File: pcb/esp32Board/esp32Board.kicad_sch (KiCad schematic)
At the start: 35 parts, among them J1 ESPProgJTAG_RX, J10 USB_C_Receptacle_USB2.0, J11 Conn_01x14_Female, J3 ESPProgUART_RX, J4 CAN, J5 UART2, J6 I2C, J7 InputOnly, J8 PWR, J9 GND, SW1 SW_Push, SW2 SW_Push_SPDT, SW3 SW_Push_SPDT, SW4 SW_Push_SPDT, U1 ESP32-WROOM-32D, U3 XC6209

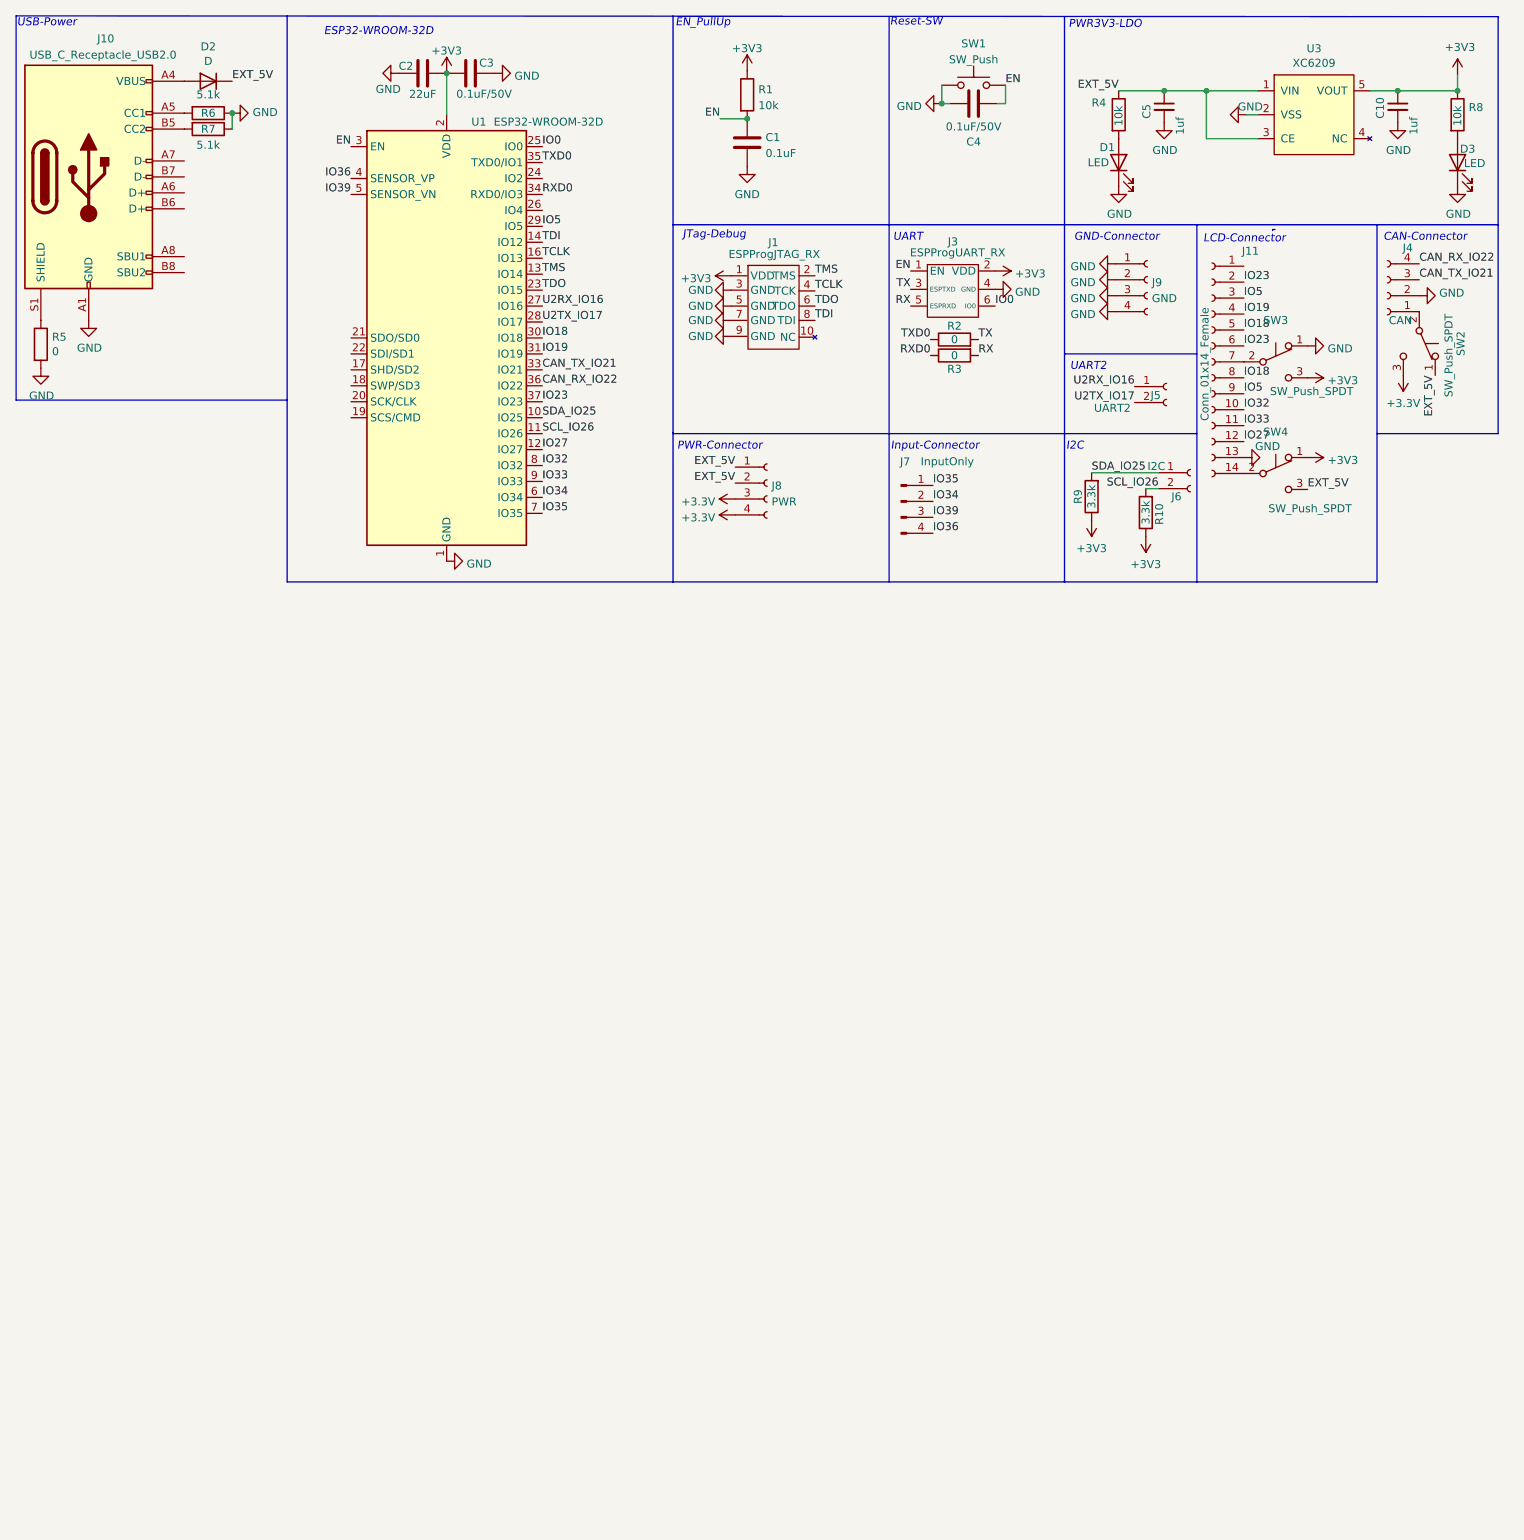
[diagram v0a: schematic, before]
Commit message: 改成竖的，论文好看
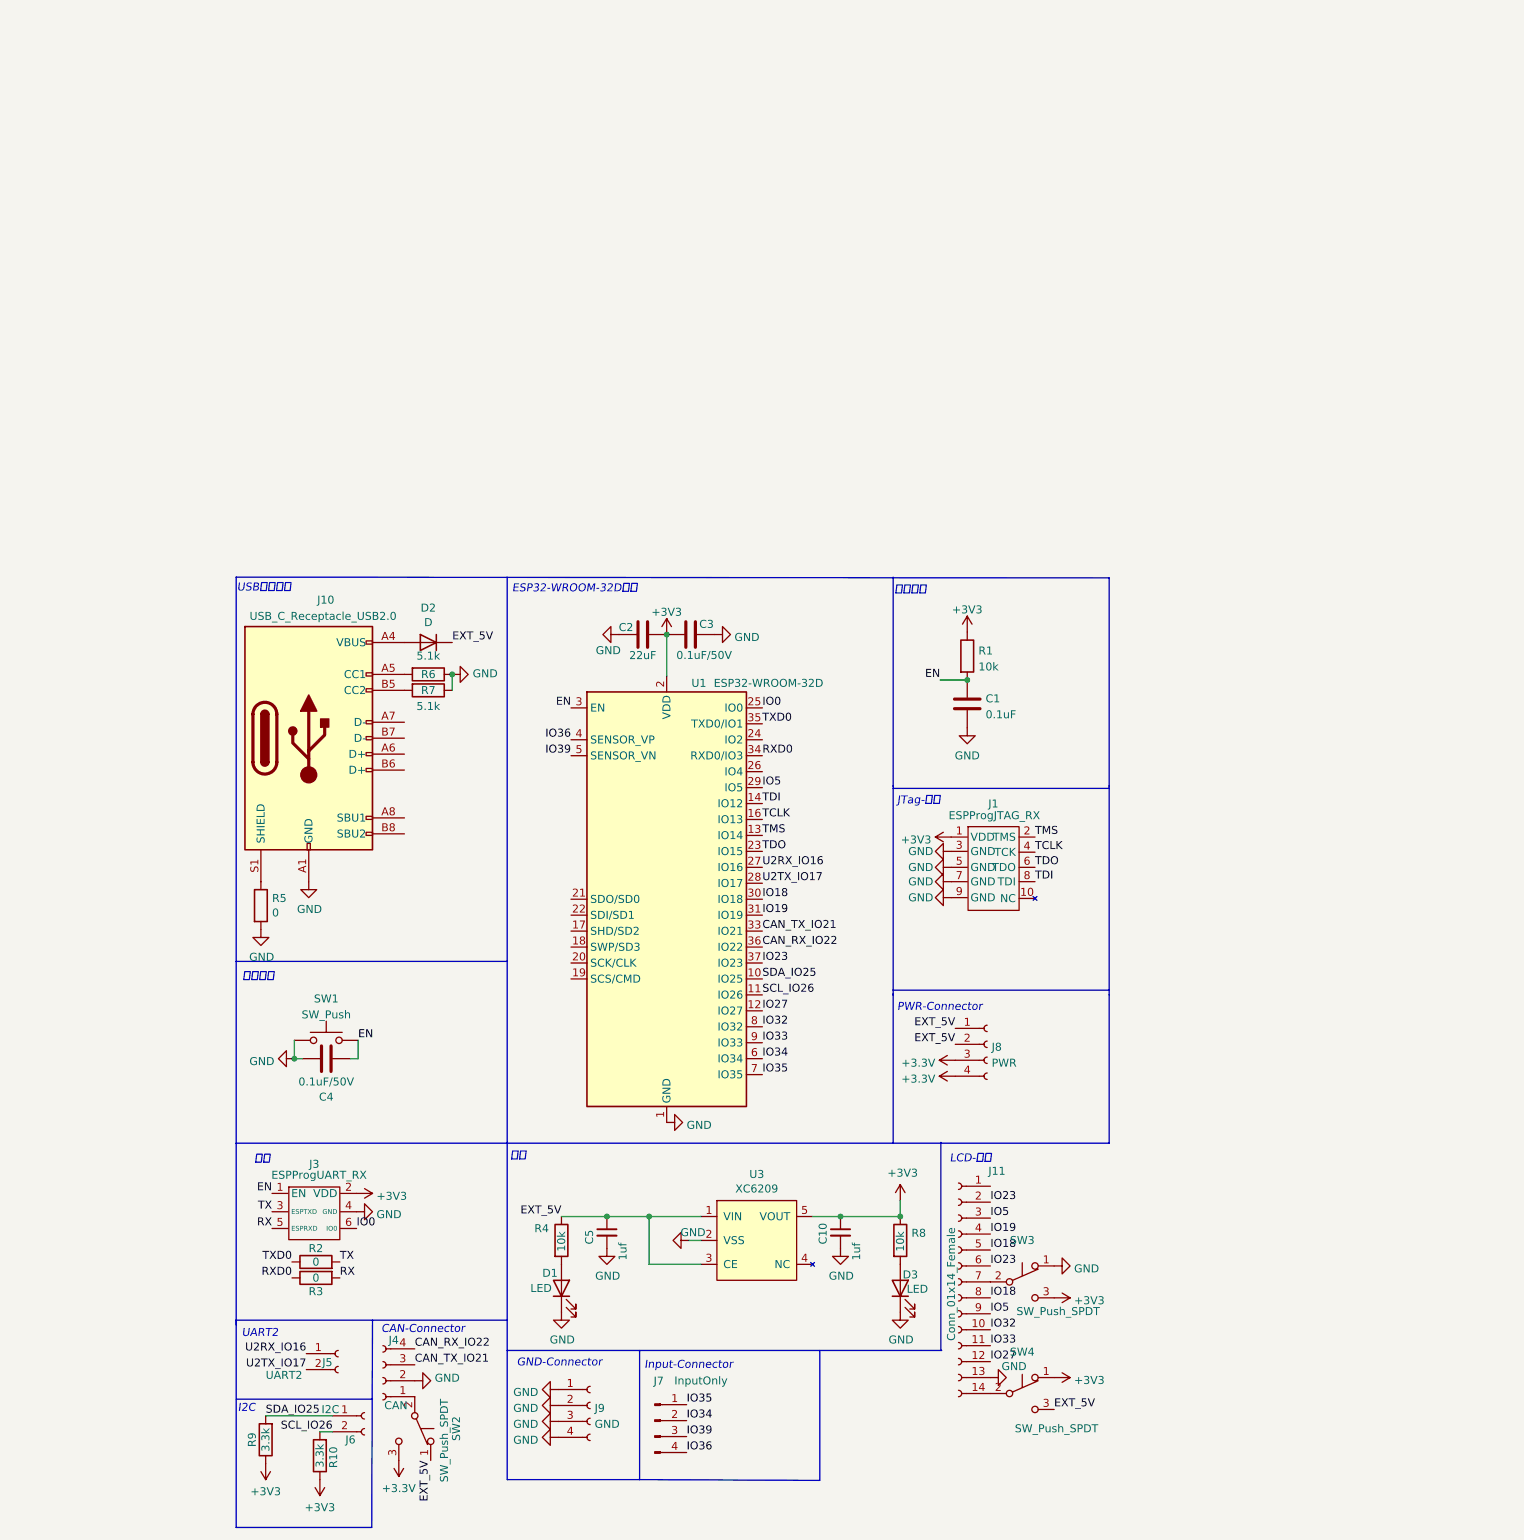
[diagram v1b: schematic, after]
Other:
- note added: "ESP32-WROOM-32D模块"
- note added: "JTag-调试"
- note added: "LCD-屏幕"
- note added: "USB电源输入"
- note added: "串口"
- note added: "复位上拉"
- note added: "复位开关"
- note added: "电源"
- note removed: "EN_PullUp"
- note removed: "ESP32-WROOM-32D"
- note removed: "JTag-Debug"
- note removed: "LCD-Connector"
- note removed: "PWR3V3-LDO"
- note removed: "Reset-SW"
- note removed: "UART"
- note removed: "USB-Power"
- moved on the sheet: C1, C10, C2, C3, C4, C5, D1, D2, D3, J1, J10, J11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
